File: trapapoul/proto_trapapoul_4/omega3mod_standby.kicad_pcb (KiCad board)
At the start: 2 copper layers, 110 x 50 mm, 116 parts, among them J101 HEADER_3x2, J401 HEADER_2, J402 HEADER_2, J403 HEADER_2, J410 HEADER_4, J730 HEADER_2, J801 HEADER_1, J802 HEADER_1, J901 HEADER_6, J902 HEADER_6, Q811 PBSS4320, Q812 PBSS5350, Q821 PBSS4320, Q822 PBSS5350, Q900 PBSS4320, U100 ATMEGA328P-A, U201 MCP7940, U500 MIC5205, U510 MIC5205, U520 MIC5205, U601 A3144, U602 A3144, U603 A3144, U604 A3144, U715 TLV431-DBZ, U830 MCP601-SOT, U900 PCF8574, X104 16M, X201 32.768K

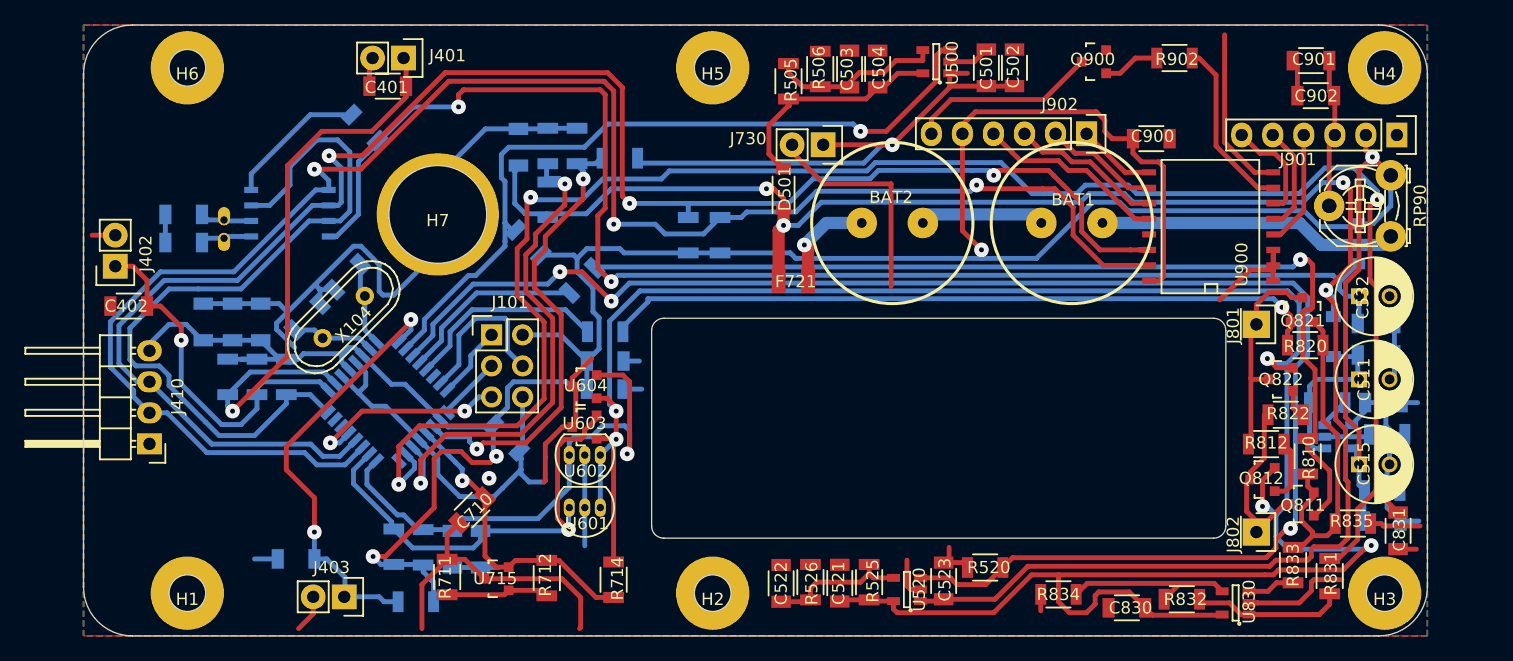
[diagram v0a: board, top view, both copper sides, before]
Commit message: prototrapapoul4 un peu retouché
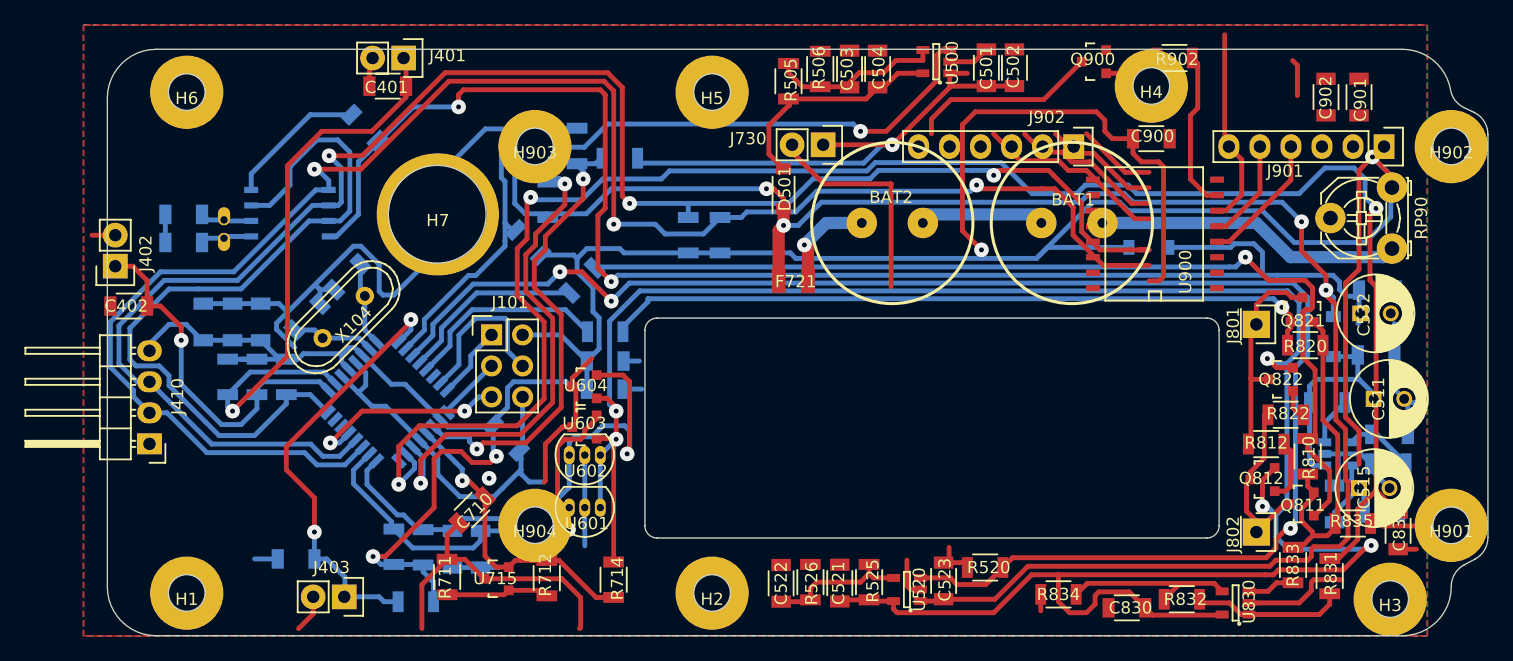
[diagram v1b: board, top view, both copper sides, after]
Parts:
- added H901: hole, gdi:3mm_screw, F.Cu at (211.9, 91.0)
- added H902: hole, gdi:3mm_screw, F.Cu at (211.9, 60.0)
- added H903: hole, gdi:3mm_screw, F.Cu at (136.9, 60.0)
- added H904: hole, gdi:3mm_screw, F.Cu at (136.9, 91.0)
- moved H4 19.2 mm to (187.4, 55.0)
- moved D530 17.1 mm to (187.2, 68.2), turned to 180 degrees
- moved C901 4.94 mm to (204.4, 55.9), turned to 270 degrees
- moved U900 4.64 mm to (187.7, 67.1)
- moved C512 4.14 mm to (202.4, 89.2), turned to 90 degrees
- moved C531 2.73 mm to (205.9, 71.7)
- moved C513 2.65 mm to (206.9, 83.5)
- moved R511 2.40 mm to (206.8, 85.9)
- moved H5 2.00 mm to (151.4, 55.5)
- moved H6 2.00 mm to (108.5, 55.5)
- moved C511 2.00 mm to (205.6, 80.6)
- moved C515 1.94 mm to (204.4, 87.9)
- moved R512 1.70 mm to (206.3, 89.8)
- moved J902 1.48 mm to (181.1, 60.0)
- moved J901 1.42 mm to (206.4, 60.0)
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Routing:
- net Net-(J902-Pad4): track 15.6 -> 0.00 mm
- net Net-(C901-Pad2): track 12.3 -> 0.00 mm
- net VCC: track 254.9 -> 265.4 mm
- net quadA: track 38.1 -> 27.7 mm, vias 1 -> 0
- net quadB: track 42.1 -> 32.5 mm
- net (no net): track 0.00 -> 9.46 mm, vias 0 -> 1
- net V_rtc: track 115.1 -> 123.0 mm
- net Net-(J901-Pad6): track 8.69 -> 15.7 mm
- net V_bat: track 152.4 -> 145.5 mm
- net Net-(C511-Pad1): track 14.5 -> 18.0 mm
- net Net-(Q900-Pad1): track 4.67 -> 1.15 mm
- net Net-(J902-Pad3): track 12.6 -> 15.6 mm
- net Net-(J902-Pad2): track 9.49 -> 12.6 mm
- net Net-(J902-Pad1): track 6.43 -> 9.49 mm
- net Net-(C513-Pad1): track 12.4 -> 9.86 mm
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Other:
- board size 110 x 50 mm -> 113 x 48 mm
